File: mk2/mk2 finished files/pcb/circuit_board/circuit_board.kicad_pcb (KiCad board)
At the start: 2 copper layers, 66 x 58.9 mm, 14 parts, among them J1 1x2 Header, J2 1x2 Header, Q1 IRLZ44N, SW1 Momentary

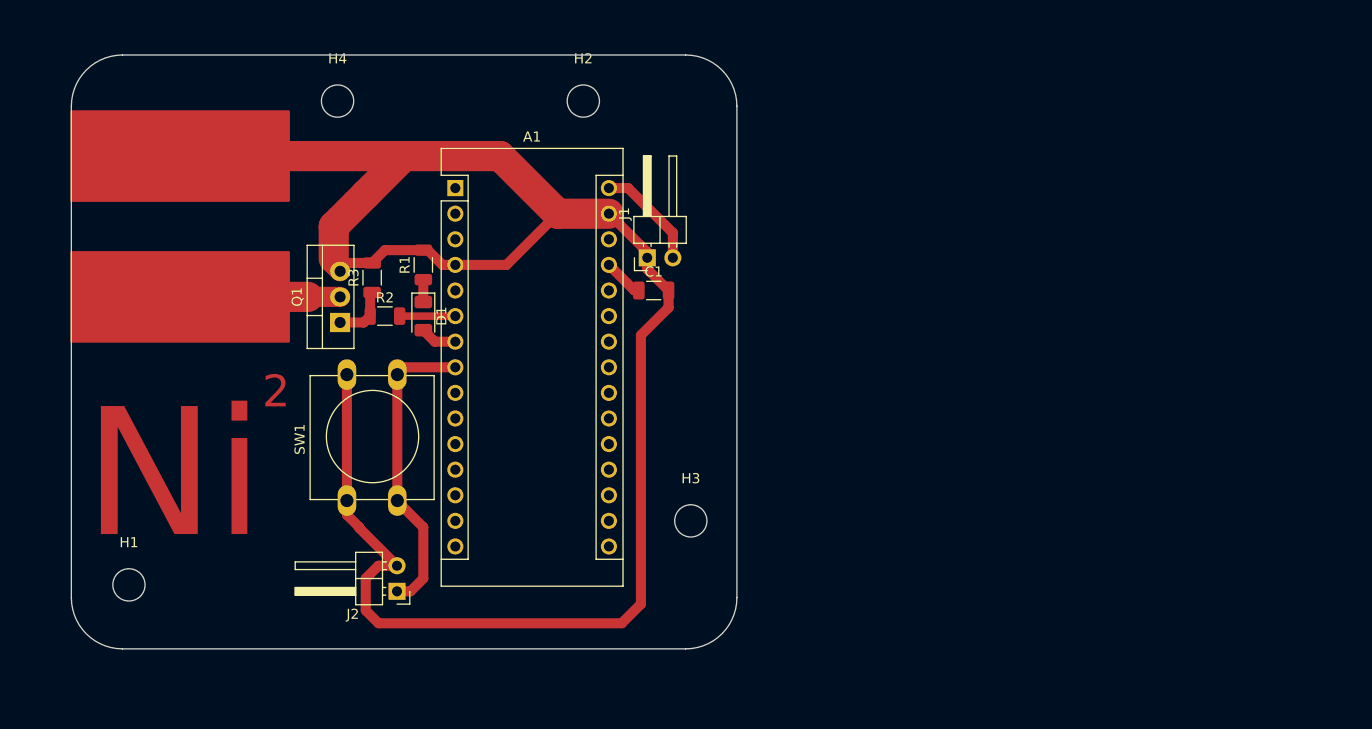
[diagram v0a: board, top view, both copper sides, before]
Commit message: PCB Updates
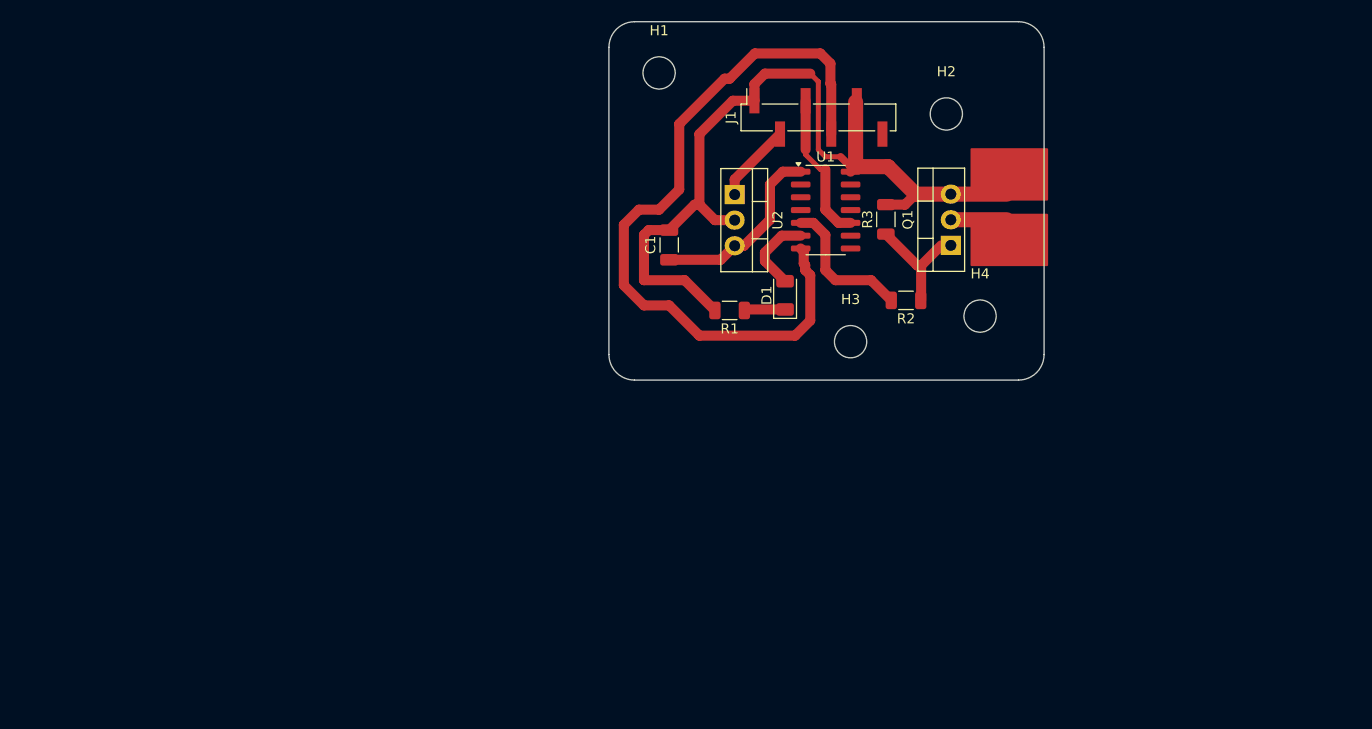
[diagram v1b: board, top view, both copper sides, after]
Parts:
- removed A1: Arduino Nano, Module:Arduino_Nano
- removed J2: 1x2 Header, Connector_PinHeader_2.54mm:PinHeader_1x02_P2.54mm_Horizontal
- removed SW1: Momentary, Button_Switch_THT:SW_PUSH-12mm
- added U1: ATtiny1614-SS, Package_SO:SOIC-14_3.9x8.7mm_P1.27mm, F.Cu at (181.5, 88.5)
- added U2: L7805, Package_TO_SOT_THT:TO-220-3_Vertical, F.Cu at (172.5, 87.0)
- J1: value 1x2 Header -> 2x3 Header; footprint Connector_PinHeader_2.54mm:PinHeader_1x02_P2.54mm_Horizontal -> Connector_PinHeader_2.54mm:PinHeader_1x06_P2.54mm_Vertical_SMD_Pin1Right
- moved H1 73.1 mm to (165.0, 74.9)
- moved H4 67.2 mm to (196.8, 99.1)
- moved Q1 61.1 mm to (193.9, 92.0)
- moved R2 51.7 mm to (189.5, 97.5), turned to 180 degrees
- moved R3 51.3 mm to (187.5, 89.5)
- moved H2 36.0 mm to (193.5, 79.0)
- moved D1 36.0 mm to (177.5, 97.0), turned to 90 degrees
- moved R1 30.7 mm to (172.0, 98.5), turned to 180 degrees
- moved H3 23.8 mm to (184.0, 101.6)
- moved J1 22.0 mm to (180.8, 79.3)
- moved C1 4.77 mm to (166.0, 92.0), turned to 90 degrees
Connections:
- C1 pad 2: +28V -> Net-(J1-Pin_1)
- J1 pad 1: +28V -> Net-(J1-Pin_1)
- Q1 pad 2: +28V -> unconnected-(Q1-D-Pad2)
- Q1 pad 3: +28V -> Net-(J1-Pin_1)
- R1 pad 2: +28V -> Net-(J1-Pin_1)
- R3 pad 2: +28V -> Net-(J1-Pin_1)
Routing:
- net +28V: track 182.8 -> 0.00 mm
- net Net-(J1-Pin_1): track 0.00 -> 84.2 mm
- net Net-(J1-Pin_4): track 0.00 -> 73.5 mm
- net Net-(A1-Pad8): track 30.5 -> 0.00 mm
- net Net-(J1-Pin_3): track 0.00 -> 15.0 mm
- net Net-(U1-VCC): track 4.02 -> 18.7 mm
- net Net-(U1-PA7//D3): track 5.52 -> 14.2 mm
- net unconnected-(Q1-D-Pad2): track 0.00 -> 5.56 mm
- net Net-(Q1-G): track 5.67 -> 11.1 mm
- net Net-(D1-A): track 3.65 -> 7.92 mm
- net Net-(J1-Pin_2): track 10.7 -> 7.86 mm
- net Net-(D1-K): track 2.22 -> 4.08 mm
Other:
- board size 66 x 58.9 mm -> 43.2 x 35.6 mm
- board text removed: "2"
- board text removed: "Ni"

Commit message: Circuit Board Edits
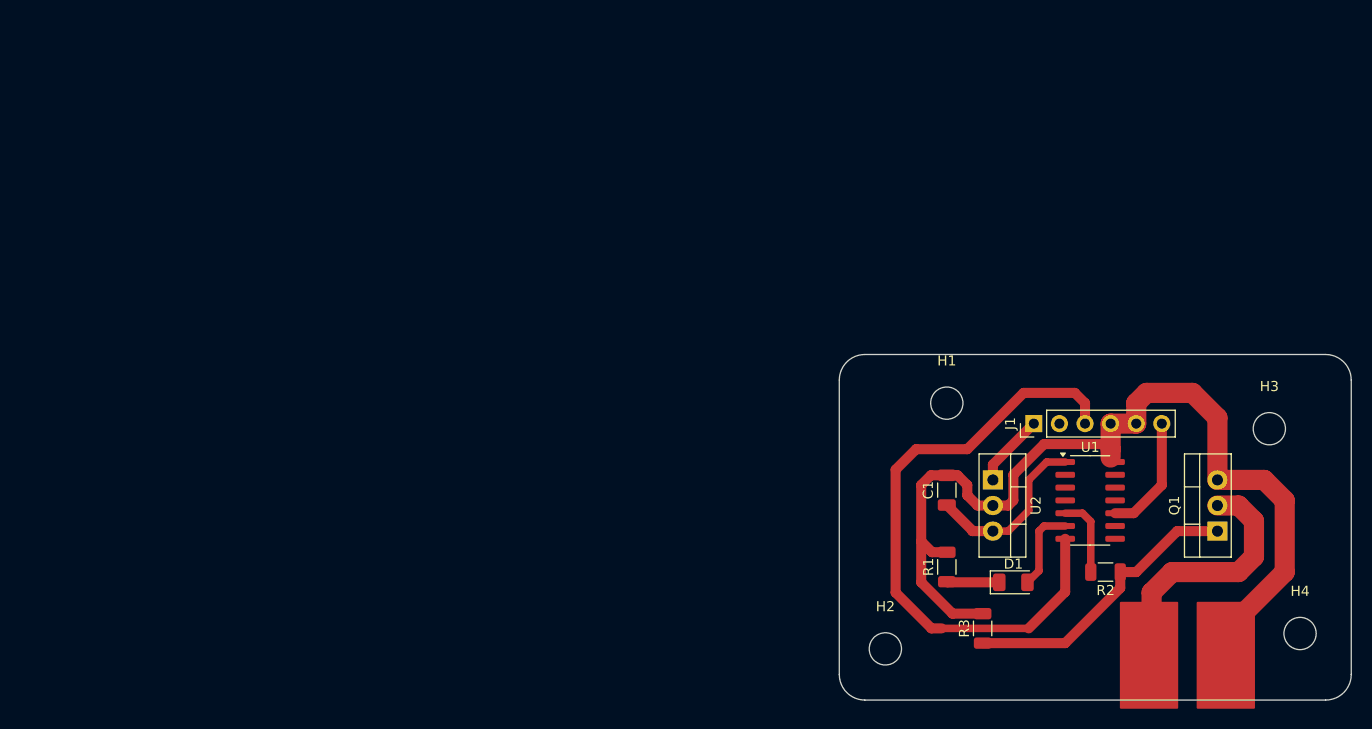
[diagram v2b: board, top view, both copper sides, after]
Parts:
- J1: footprint Connector_PinHeader_2.54mm:PinHeader_1x06_P2.54mm_Vertical_SMD_Pin1Right -> Connector_PinHeader_2.54mm:PinHeader_1x06_P2.54mm_Vertical
- U1: value ATtiny1614-SS -> ATtiny1614
- moved H2 53.4 mm to (187.5, 132.1)
- moved H4 44.7 mm to (228.6, 130.6)
- moved H1 43.5 mm to (193.5, 107.7)
- moved H3 42.4 mm to (225.6, 110.2)
- moved R3 41.7 mm to (197.1, 130.0)
- moved U1 39.0 mm to (207.8, 117.3)
- moved Q1 38.8 mm to (220.4, 120.4)
- moved U2 38.2 mm to (198.1, 115.3)
- moved J1 37.1 mm to (202.2, 109.7)
- moved C1 36.8 mm to (193.5, 116.3)
- moved D1 36.4 mm to (200.2, 125.5), turned to 0 degrees
- moved R2 33.4 mm to (209.3, 124.5)
- moved R1 33.3 mm to (193.5, 124.0), turned to 90 degrees
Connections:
- C1 pad 2: Net-(J1-Pin_1) -> Net-(J1-Pin_4)
- J1 pad 2: Net-(J1-Pin_2) -> unconnected-(J1-Pin_2-Pad2)
- J1 pad 5: Net-(J1-Pin_1) -> Net-(J1-Pin_4)
- J1 pad 6: unconnected-(J1-Pin_6-Pad6) -> Net-(J1-Pin_6)
- Q1 pad 3: Net-(J1-Pin_1) -> Net-(J1-Pin_4)
- R1 pad 2: Net-(J1-Pin_1) -> Net-(J1-Pin_4)
- R3 pad 2: Net-(J1-Pin_1) -> Net-(J1-Pin_4)
- U1 pad 10: Net-(J1-Pin_3) -> Net-(J1-Pin_6)
- U1 pad 14: Net-(J1-Pin_1) -> Net-(J1-Pin_4)
- U1 pad 7: Net-(J1-Pin_4) -> Net-(J1-Pin_3)
- U2 pad 1: Net-(J1-Pin_2) -> Net-(J1-Pin_1)
- U2 pad 2: Net-(J1-Pin_1) -> Net-(J1-Pin_4)
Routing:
- net Net-(J1-Pin_1): track 84.2 -> 7.27 mm
- net Net-(J1-Pin_3): track 15.0 -> 61.7 mm
- net Net-(J1-Pin_4): track 73.5 -> 91.3 mm
- net Net-(Q1-G): track 11.1 -> 28.8 mm
- net unconnected-(Q1-D-Pad2): track 5.56 -> 20.5 mm
- net Net-(J1-Pin_6): track 0.00 -> 11.9 mm
- net Net-(J1-Pin_2): track 7.86 -> 0.00 mm
- net Net-(U1-PA7//D3): track 14.2 -> 7.90 mm
- net Net-(U1-VCC): track 18.7 -> 17.5 mm
- net Net-(D1-K): track 4.08 -> 5.23 mm
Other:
- board size 43.2 x 35.6 mm -> 50.8 x 34.3 mm
